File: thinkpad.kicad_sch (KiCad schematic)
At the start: 125 parts, among them J1 Conn_01x06_MountingPin, J2 Conn_01x20_Socket, J3 Conn_01x06_Socket, SW1 SW_Push, U1 Raspberry_Pi_Pico

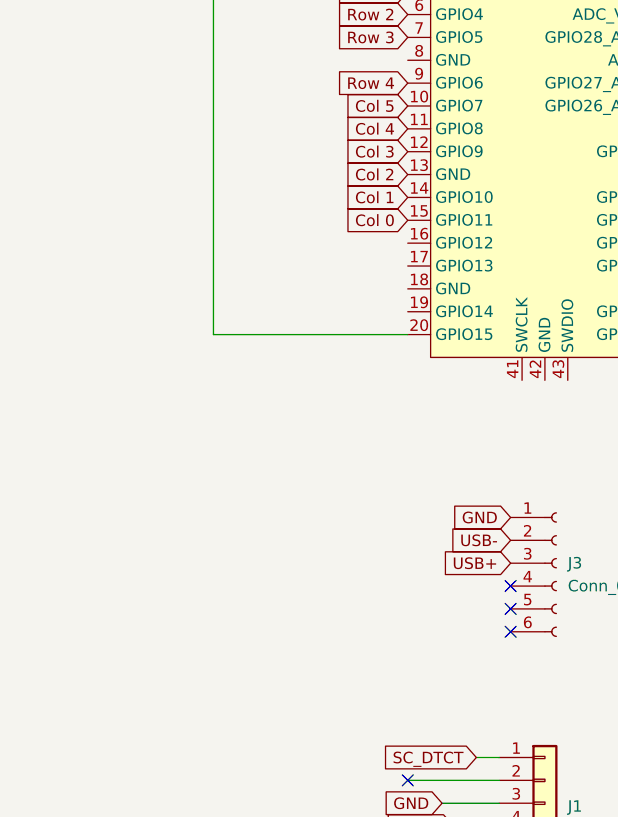
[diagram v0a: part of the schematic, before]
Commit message: Improvements
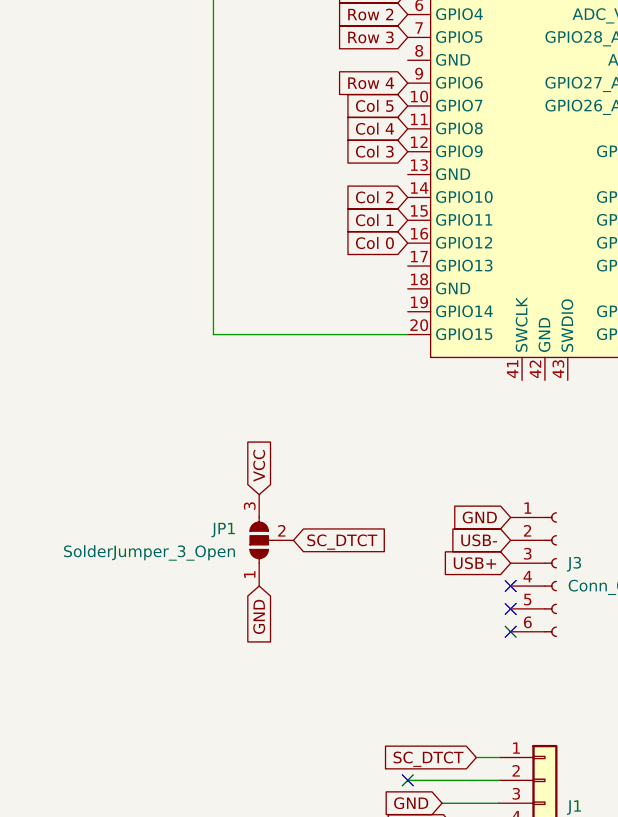
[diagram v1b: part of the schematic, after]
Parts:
- added JP1: SolderJumper_3_Open, Jumper:SolderJumper-3_P1.3mm_Open_Pad1.0x1.5mm_NumberLabels, symbol Jumper:SolderJumper_3_Open
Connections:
- net Col 0: now also U1.16 (GPIO12); no longer U1.15 (GPIO11)
- net Col 1: now also U1.15 (GPIO11); no longer U1.14 (GPIO10)
- net Col 2: now also U1.14 (GPIO10); no longer U1.13 (GND)
- net GND: now also JP1.1 (A)
- net SC_DTCT: now also JP1.2 (C)
- net VCC: now also JP1.3 (B)
